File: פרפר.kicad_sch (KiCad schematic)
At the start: 52 parts, among them J1 JST_SH_BM03B-SRSS-TB, J2 Hirose_FH12-22S-0.5SH, J5 JST_SH_SM04B-SRSS-TB, J6 JST_SUR_SM02B-SURS-TF, J7 JST_SH_BM03B-SRSS-TB

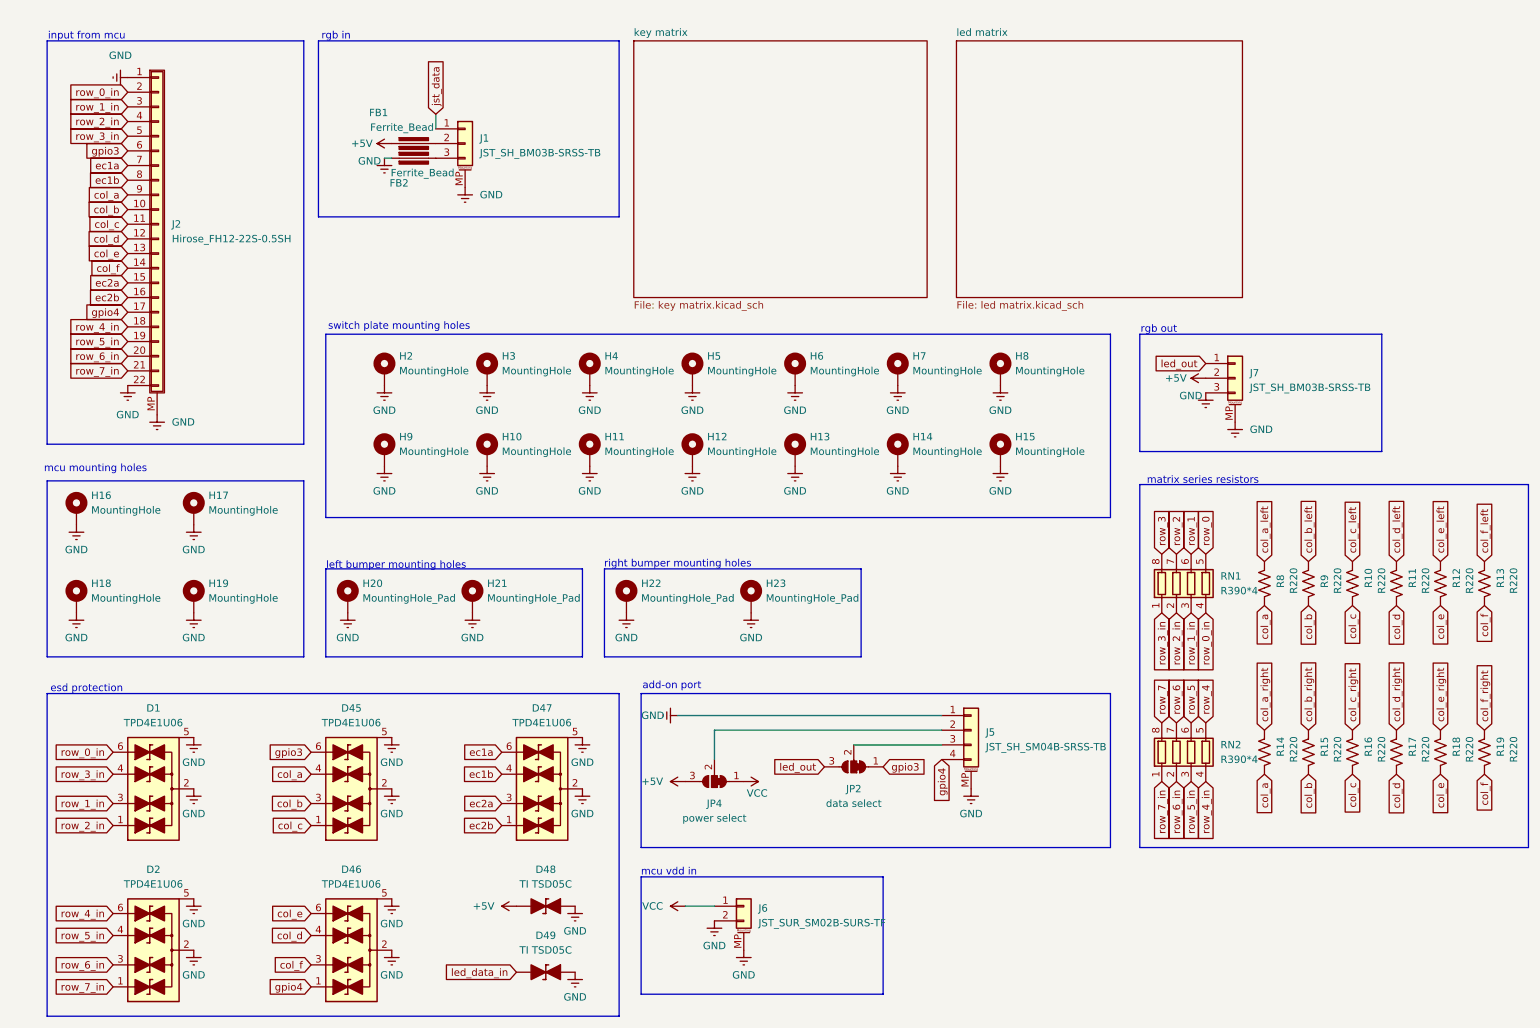
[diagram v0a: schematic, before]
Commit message: v2 final ready to order
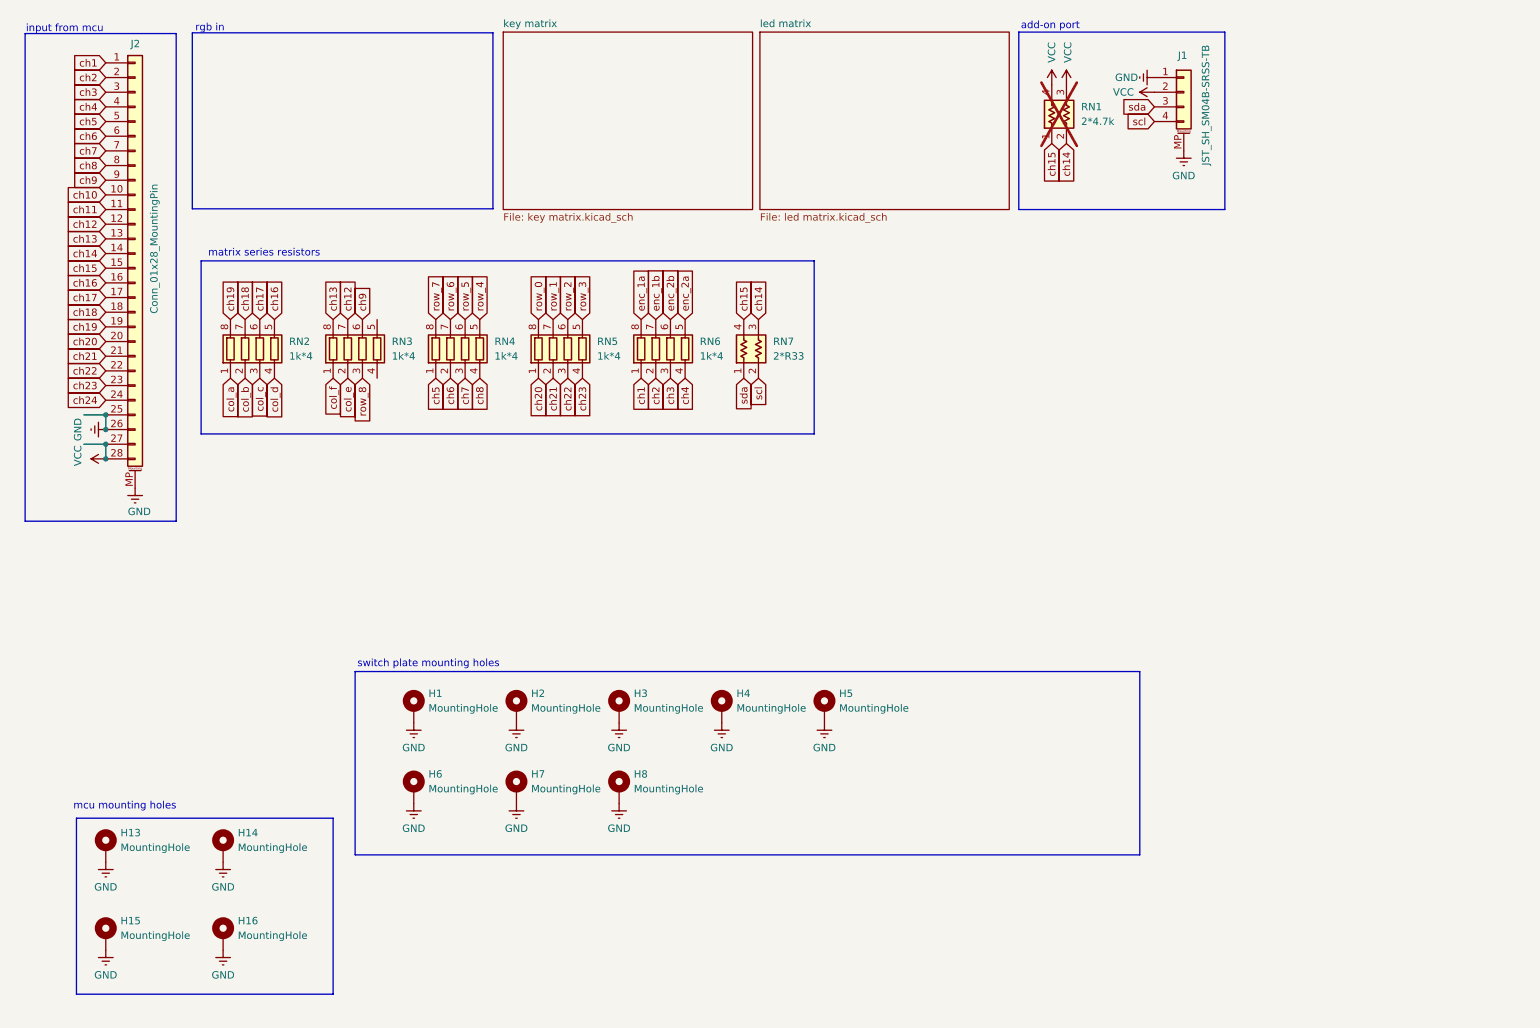
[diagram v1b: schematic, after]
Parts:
- removed D1, D2, D45, D46, D47: TPD4E1U06, PCM_Package_TO_SOT_SMD_AKL:SOT-363_SC-70-6, symbol coquette_symbols:TPD4E1U06
- removed D48, D49: TI TSD05C, PCM_Diode_SMD_AKL:D_SOD-323_TVS, symbol PCM_Diode_TVS_AKL:D_TVS_Bidirectional_Generic
- removed FB1, FB2: Ferrite_Bead, PCM_Ferrite_SMD_AKL:Ferrite_0805_2012Metric, symbol PCM_Device_AKL:Ferrite_Bead
- removed H12, H13, H14, H15, H7, H8: MountingHole, MountingHole:MountingHole_3.2mm_M3_DIN965_Pad, symbol Mechanical:MountingHole_Pad
- removed H20, H21, H22, H23: MountingHole_Pad, MountingHole:MountingHole_2.2mm_M2_DIN965_Pad, symbol Mechanical:MountingHole_Pad
- removed J1, J7: JST_SH_BM03B-SRSS-TB, Connector_JST:JST_SH_BM03B-SRSS-TB_1x03-1MP_P1.00mm_Vertical, symbol Connector_Generic_MountingPin:Conn_01x03_MountingPin
- removed J6: JST_SUR_SM02B-SURS-TF, Connector_JST:JST_SUR_SM02B-SURS-TF_1x02-1MP_P0.80mm_Horizontal, symbol Connector_Generic_MountingPin:Conn_01x02_MountingPin
- removed JP2: data select, Jumper:SolderJumper-3_P1.3mm_Bridged12_RoundedPad1.0x1.5mm, symbol Jumper:SolderJumper_3_Bridged12
- removed JP4: power select, Jumper:SolderJumper-3_P1.3mm_Bridged12_RoundedPad1.0x1.5mm, symbol Jumper:SolderJumper_3_Bridged12
- removed R10, R11, R12, R13, R14, R15, R16, R17, R18, R19, R8, R9: R220, Resistor_SMD:R_0805_2012Metric, symbol Device:R_US
- added RN1: 2*4.7k, Resistor_SMD:R_Array_Convex_2x0402, symbol PCM_Resistor_US_AKL:R_2x0603_Concave
- added RN2, RN3, RN6: 1k*4, PCM_Resistor_SMD_AKL:R_Array_Concave_4x0603, symbol PCM_Resistor_AKL:R_4x0603_Concave
- added RN7: 2*R33, PCM_Resistor_SMD_AKL:R_Array_Concave_2x0603, symbol PCM_Resistor_US_AKL:R_2x0603_Concave
- H1: renamed from H2; footprint MountingHole:MountingHole_3.2mm_M3_DIN965_Pad -> MountingHole:MountingHole_2.2mm_M2_DIN965_Pad
- H2: renamed from H16; footprint MountingHole:MountingHole_3.2mm_M3_DIN965_Pad -> MountingHole:MountingHole_2.2mm_M2_DIN965_Pad
- H3: renamed from H18; footprint MountingHole:MountingHole_3.2mm_M3_DIN965_Pad -> MountingHole:MountingHole_2.2mm_M2_DIN965_Pad
- H4: renamed from H17; footprint MountingHole:MountingHole_3.2mm_M3_DIN965_Pad -> MountingHole:MountingHole_2.2mm_M2_DIN965_Pad
- H5: renamed from H19; footprint MountingHole:MountingHole_3.2mm_M3_DIN965_Pad -> MountingHole:MountingHole_2.2mm_M2_DIN965_Pad
- H6: renamed from H9; footprint MountingHole:MountingHole_3.2mm_M3_DIN965_Pad -> MountingHole:MountingHole_2.2mm_M2_DIN965_Pad
- H7: renamed from H10; footprint MountingHole:MountingHole_3.2mm_M3_DIN965_Pad -> MountingHole:MountingHole_2.2mm_M2_DIN965_Pad
- H8: renamed from H11; footprint MountingHole:MountingHole_3.2mm_M3_DIN965_Pad -> MountingHole:MountingHole_2.2mm_M2_DIN965_Pad
- J2: value Hirose_FH12-22S-0.5SH -> Conn_01x28_MountingPin; footprint Connector_FFC-FPC:Hirose_FH12-22S-0.5SH_1x22-1MP_P0.50mm_Horizontal -> coquette_footprints:FFC-28; symbol Connector_Generic_Shielded:Conn_01x22_Shielded -> Connector_Generic_MountingPin:Conn_01x28_MountingPin
- RN4: renamed from RN1; value R390*4 -> 1k*4
- RN5: renamed from RN2; value R390*4 -> 1k*4
- renumbered H3 to H13, H4 to H14, H5 to H15, H6 to H16, J5 to J1
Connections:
- net GND: now also J2.25 (Pin_25), J2.26 (Pin_26); no longer J2.1 (Pin_1), J2.22 (Pin_22)
- net VCC: now also J1.2 (Pin_2), J2.27 (Pin_27), J2.28 (Pin_28), RN1.3 (R2.2), RN1.4 (R1.2)
- net col_a: now also RN2.1 (R1.1); no longer J2.9 (Pin_9)
- net col_b: now also RN2.2 (R2.1); no longer J2.10 (Pin_10)
- net col_c: now also RN2.3 (R3.1); no longer J2.11 (Pin_11)
- net col_d: now also RN2.4 (R4.1); no longer J2.12 (Pin_12)
- net col_e: now also RN3.2 (R2.1); no longer J2.13 (Pin_13)
- net col_f: now also RN3.1 (R1.1); no longer J2.14 (Pin_14)
- net row_0: now also RN5.8 (R1.2); no longer RN4.5 (R4.2)
- net row_1: now also RN5.7 (R2.2); no longer RN4.6 (R3.2)
- net row_2: now also RN5.6 (R3.2); no longer RN4.7 (R2.2)
- net row_3: now also RN5.5 (R4.2); no longer RN4.8 (R1.2)
- net row_4: now also RN4.5 (R4.2); no longer RN5.5 (R4.2)
- net row_5: now also RN4.6 (R3.2); no longer RN5.6 (R3.2)
- net row_6: now also RN4.7 (R2.2); no longer RN5.7 (R2.2)
- net row_7: now also RN4.8 (R1.2); no longer RN5.8 (R1.2)
- net sda: now reaches J1.3 (Pin_3)
- net sda: now also RN7.1 (R1.1)
- net ec1a renamed ch7
- net ch7: now also RN4.3 (R3.1)
- net ec1b renamed ch8
- net ch8: now also RN4.4 (R4.1)
- net ec2a renamed ch15
- net ch15: now also RN1.1 (R1.1), RN7.4 (R1.2)
- net ec2b renamed ch16
- net ch16: now also RN2.5 (R4.2)
- net gpio3 renamed ch6
- net ch6: now also RN4.2 (R2.1)
- net gpio4 renamed ch17
- net ch17: now also RN2.6 (R3.2); no longer J1.4 (Pin_4)
- net row_0_in renamed ch2
- net ch2: now also RN6.2 (R2.1); no longer RN4.4 (R4.1)
- net row_1_in renamed ch3
- net ch3: now also RN6.3 (R3.1); no longer RN4.3 (R3.1)
- net row_2_in renamed ch4
- net ch4: now also RN6.4 (R4.1); no longer RN4.2 (R2.1)
- net row_3_in renamed ch5
- net row_4_in renamed ch18
- net ch18: now also RN2.7 (R2.2); no longer RN5.4 (R4.1)
- net row_5_in renamed ch19
- net ch19: now also RN2.8 (R1.2); no longer RN5.3 (R3.1)
- net row_6_in renamed ch20
- net ch20: now also RN5.1 (R1.1); no longer RN5.2 (R2.1)
- net row_7_in renamed ch21
- net ch21: now also RN5.2 (R2.1); no longer RN5.1 (R1.1)
- new net ch1: J2.1 (Pin_1), RN6.1 (R1.1)
- new net ch10: J2.10 (Pin_10)
- new net ch11: J2.11 (Pin_11)
- new net ch12: J2.12 (Pin_12), RN3.7 (R2.2)
- new net ch13: J2.13 (Pin_13), RN3.8 (R1.2)
- new net ch14: J2.14 (Pin_14), RN1.2 (R2.1), RN7.3 (R2.2)
- new net ch22: J2.22 (Pin_22), RN5.3 (R3.1)
- new net ch23: J2.23 (Pin_23), RN5.4 (R4.1)
- new net ch24: J2.24 (Pin_24)
- new net ch9: J2.9 (Pin_9), RN3.6 (R3.2)
- new net enc_1a: RN6.8 (R1.2)
- new net enc_1b: RN6.7 (R2.2)
- new net enc_2a: RN6.5 (R4.2)
- new net enc_2b: RN6.6 (R3.2)
- new net row_8: RN3.3 (R3.1)
- new net scl: J1.4 (Pin_4), RN7.2 (R2.1)
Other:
- note removed: "esd protection"
- note removed: "left bumper mounting holes"
- note removed: "mcu vdd in"
- note removed: "rgb out"
- note removed: "right bumper mounting holes"
- moved on the sheet: H1, H13, H14, H15, H16, H2, H3, H4, H5, H6, H7, H8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
